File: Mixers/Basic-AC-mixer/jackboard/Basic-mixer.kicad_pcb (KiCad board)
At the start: 2 copper layers, 40 x 110 mm, 37 parts, among them J1 In, J2 Power Input, J3 In, J4 Out, J5 In, J6 In, SW1 Mute, SW2 Mute, SW3 Mute, SW4 Mute, U1 TL072

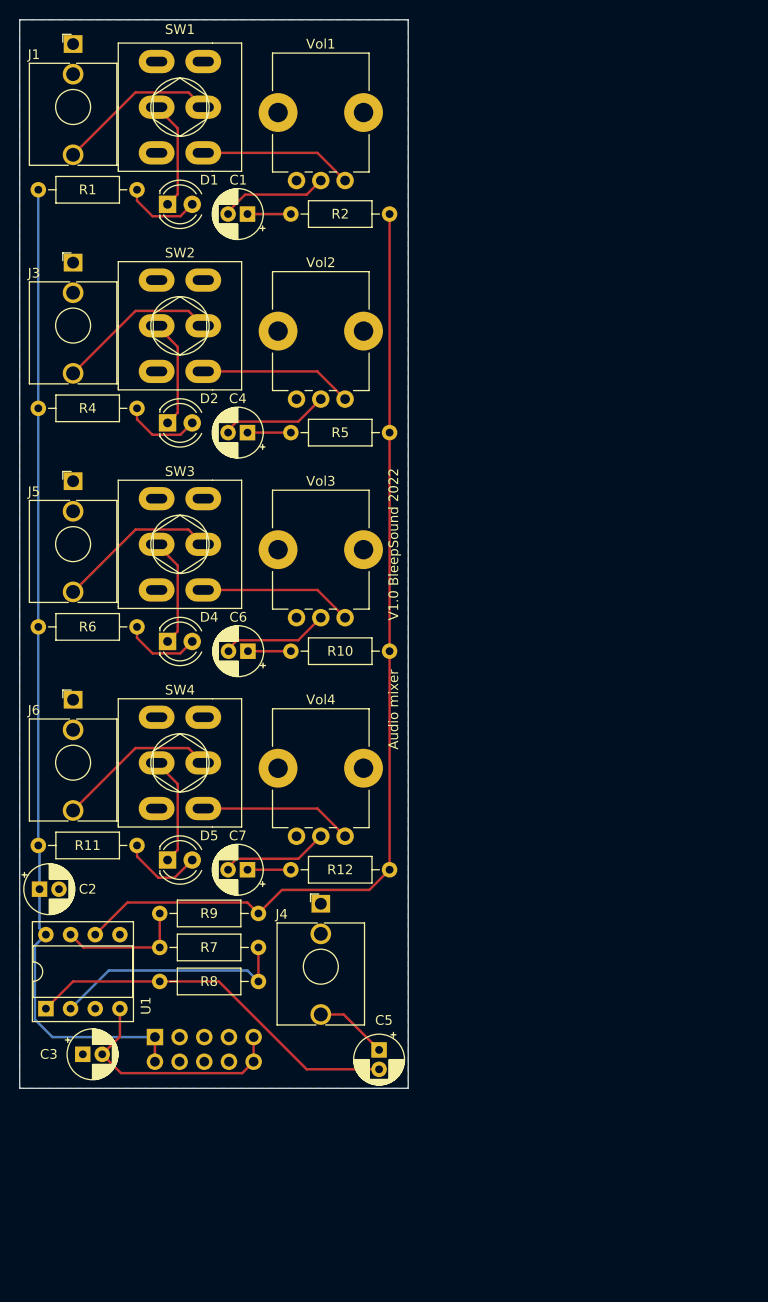
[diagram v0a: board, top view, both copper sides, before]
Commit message: output gerber for jackboard
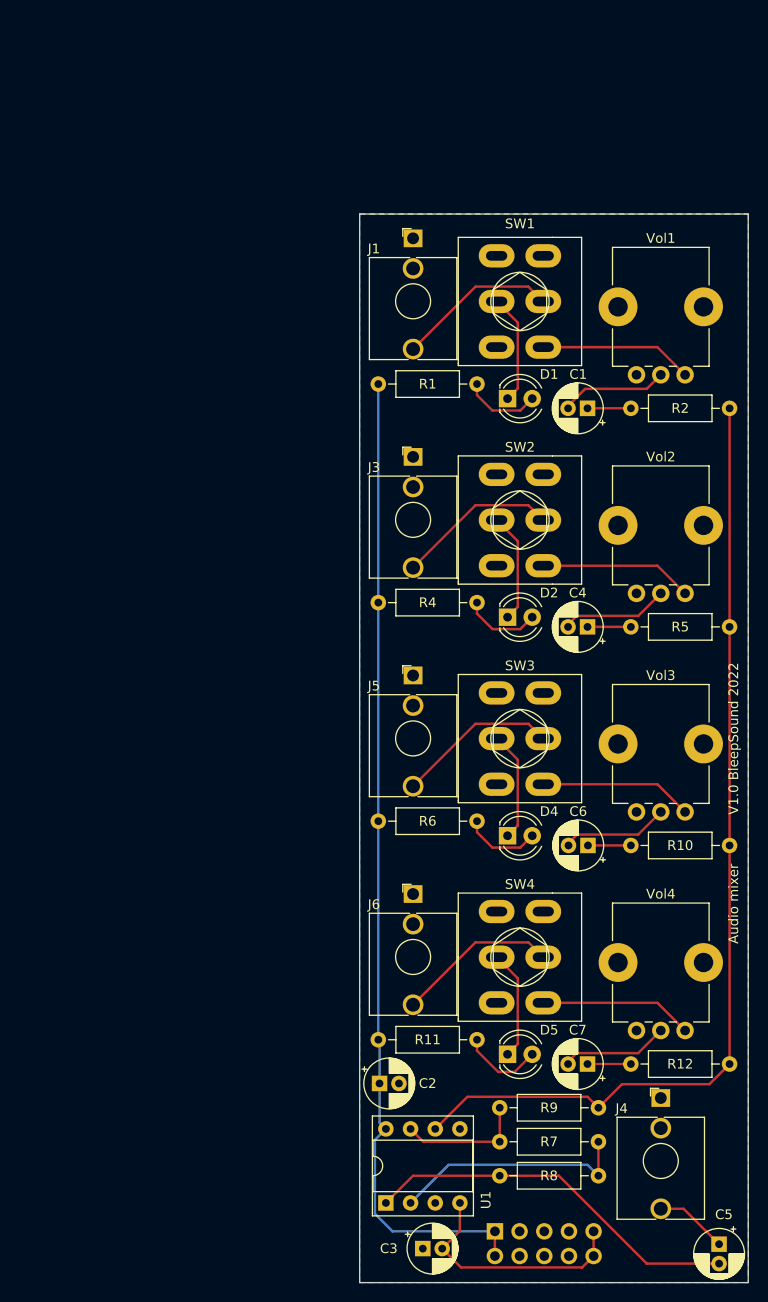
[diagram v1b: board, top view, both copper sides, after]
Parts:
- moved Vol4 40.3 mm to (98.5, 135.1)
- moved C1 40.3 mm to (88.5, 71.0)
- moved C2 40.3 mm to (67.0, 140.5)
- moved C3 40.3 mm to (71.5, 157.5)
- moved C4 40.3 mm to (88.5, 93.5)
- moved C5 40.3 mm to (102.0, 157.0)
- moved C6 40.3 mm to (88.5, 116.0)
- moved C7 40.3 mm to (88.5, 138.5)
- moved D1 40.3 mm to (80.2, 70.0)
- moved D2 40.3 mm to (80.2, 92.5)
- moved D4 40.3 mm to (80.2, 115.0)
- moved D5 40.3 mm to (80.2, 137.5)
- moved J1 40.3 mm to (70.5, 53.5)
- moved J2 40.3 mm to (78.9, 155.7)
- moved J3 40.3 mm to (70.5, 76.0)
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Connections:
- U1 pad 5: /Vgnd -> GND
